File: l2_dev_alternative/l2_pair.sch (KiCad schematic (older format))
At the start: 10 parts, among them U1102 NC7WZ17, U201 NC7WZ17, U203 NCP1529

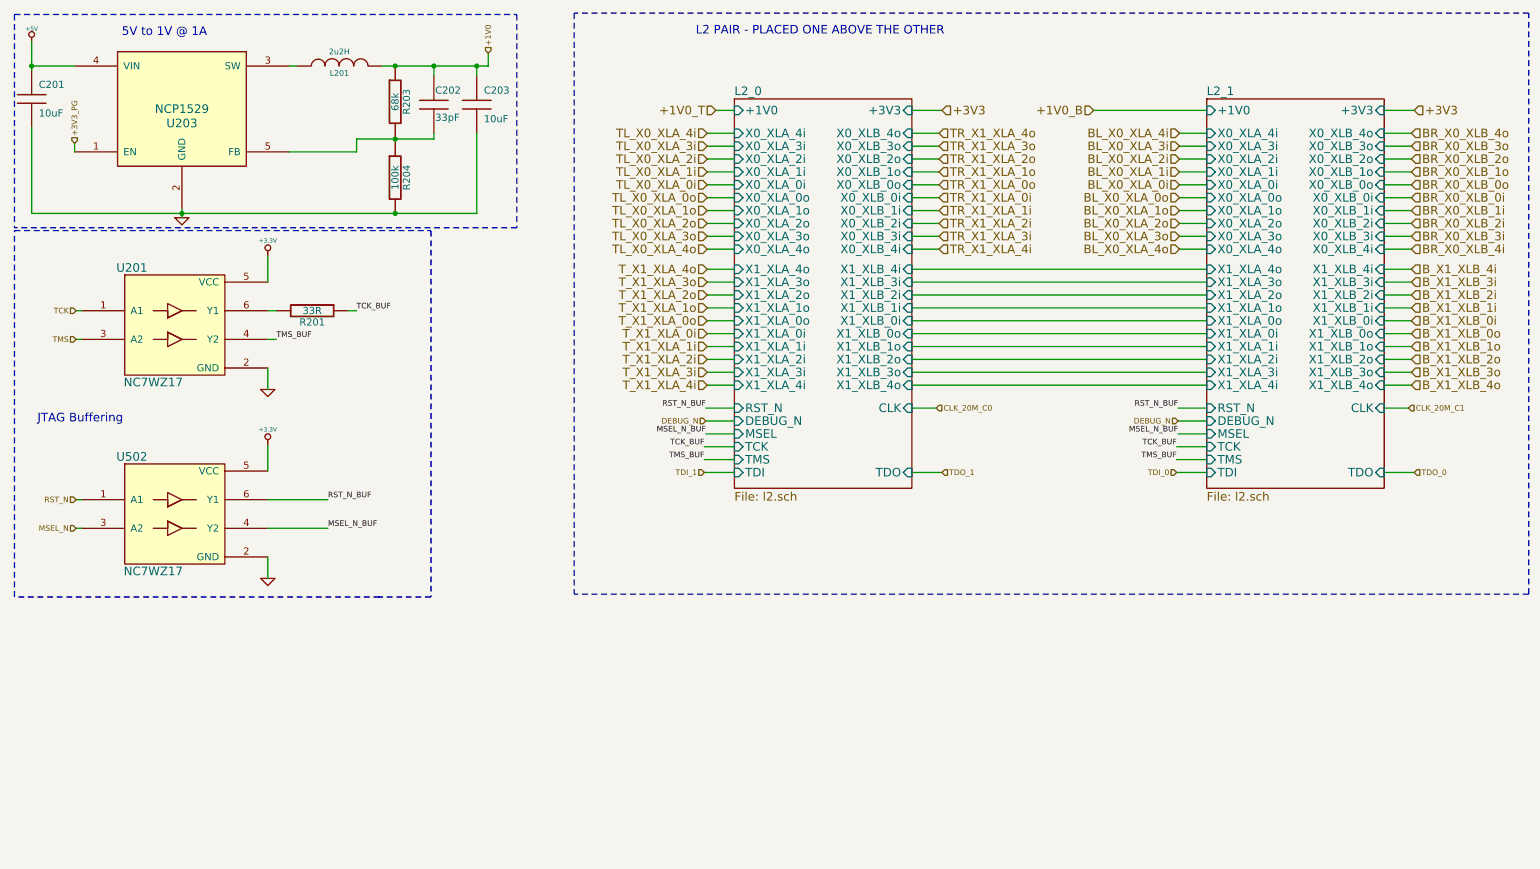
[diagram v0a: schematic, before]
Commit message: almost done!
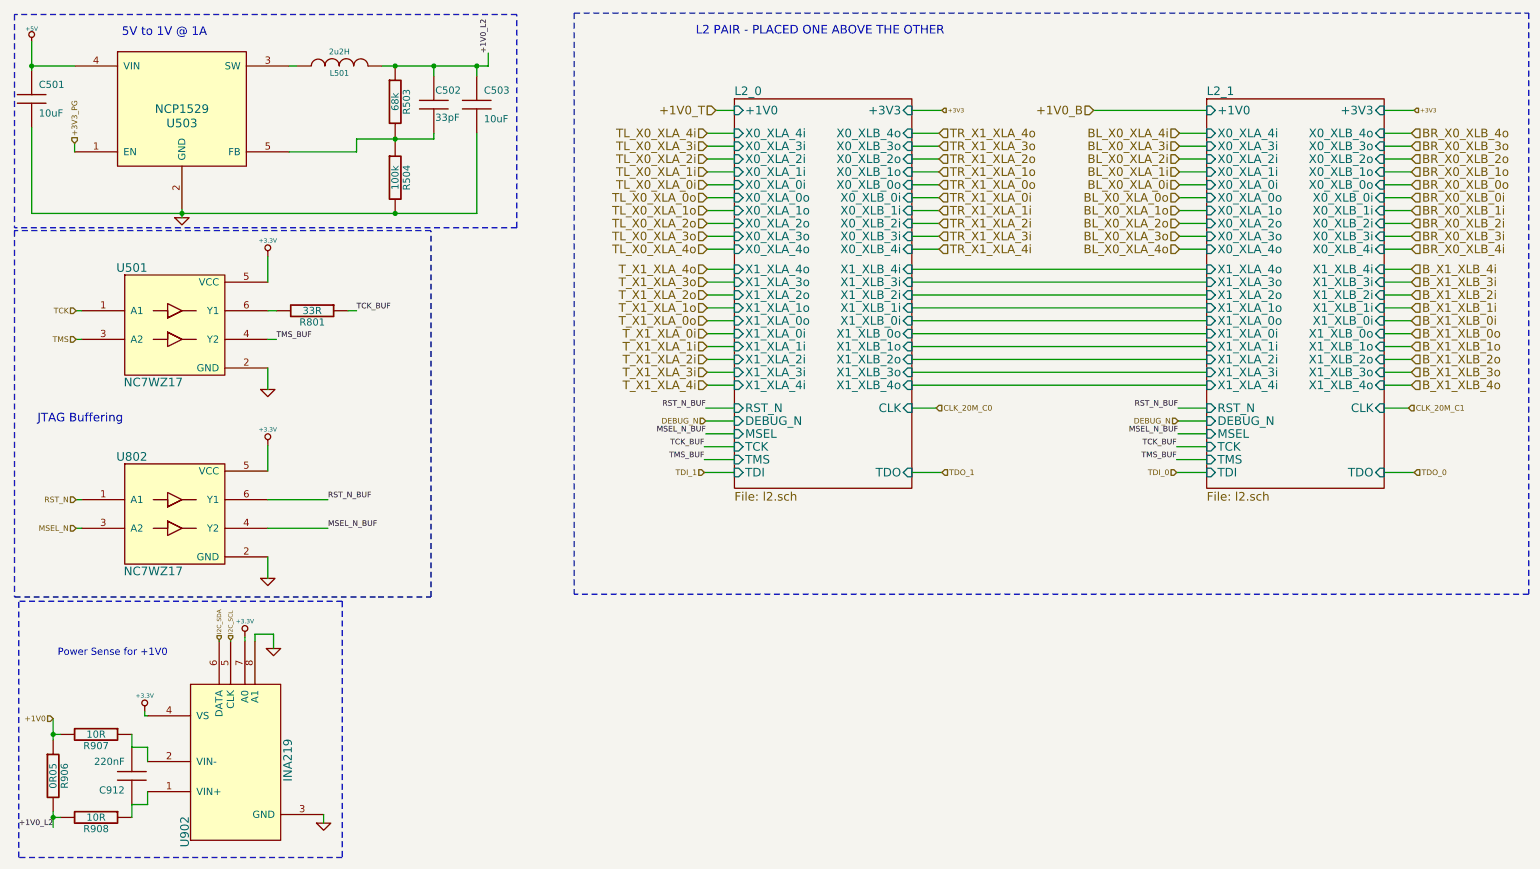
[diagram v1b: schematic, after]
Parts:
- added C312: 220nF, symbol C
- added R307, R308: 10R, symbol R
- added R606: 0R05, symbol R
- added U602: INA219, symbol INA219
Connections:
- net +1V0: now also R307.2, R606.1; no longer C202.1, C203.1, L201.2, R203.1
- net +3.3V: now also U602.4 (VS), U602.7 (A0)
- net GND: now also U602.3 (GND), U602.8 (A1)
- new net: C312.1, R308.1, U602.1 (VIN+)
- new net: C312.2, R307.1, U602.2 (VIN-)
- new net +1V0_L2: C202.1, C203.1, L201.2, R203.1, R308.2, R606.2
- new net I2C_SCL: U602.5 (CLK)
- new net I2C_SDA: U602.6 (DATA)
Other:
- note added: "Power Sense for +1V0\n"
